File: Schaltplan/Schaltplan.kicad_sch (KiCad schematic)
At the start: 9 parts, among them J2 Buck Converter, M2 Stepper_Motor_bipolar, M3 Stepper_Motor_bipolar

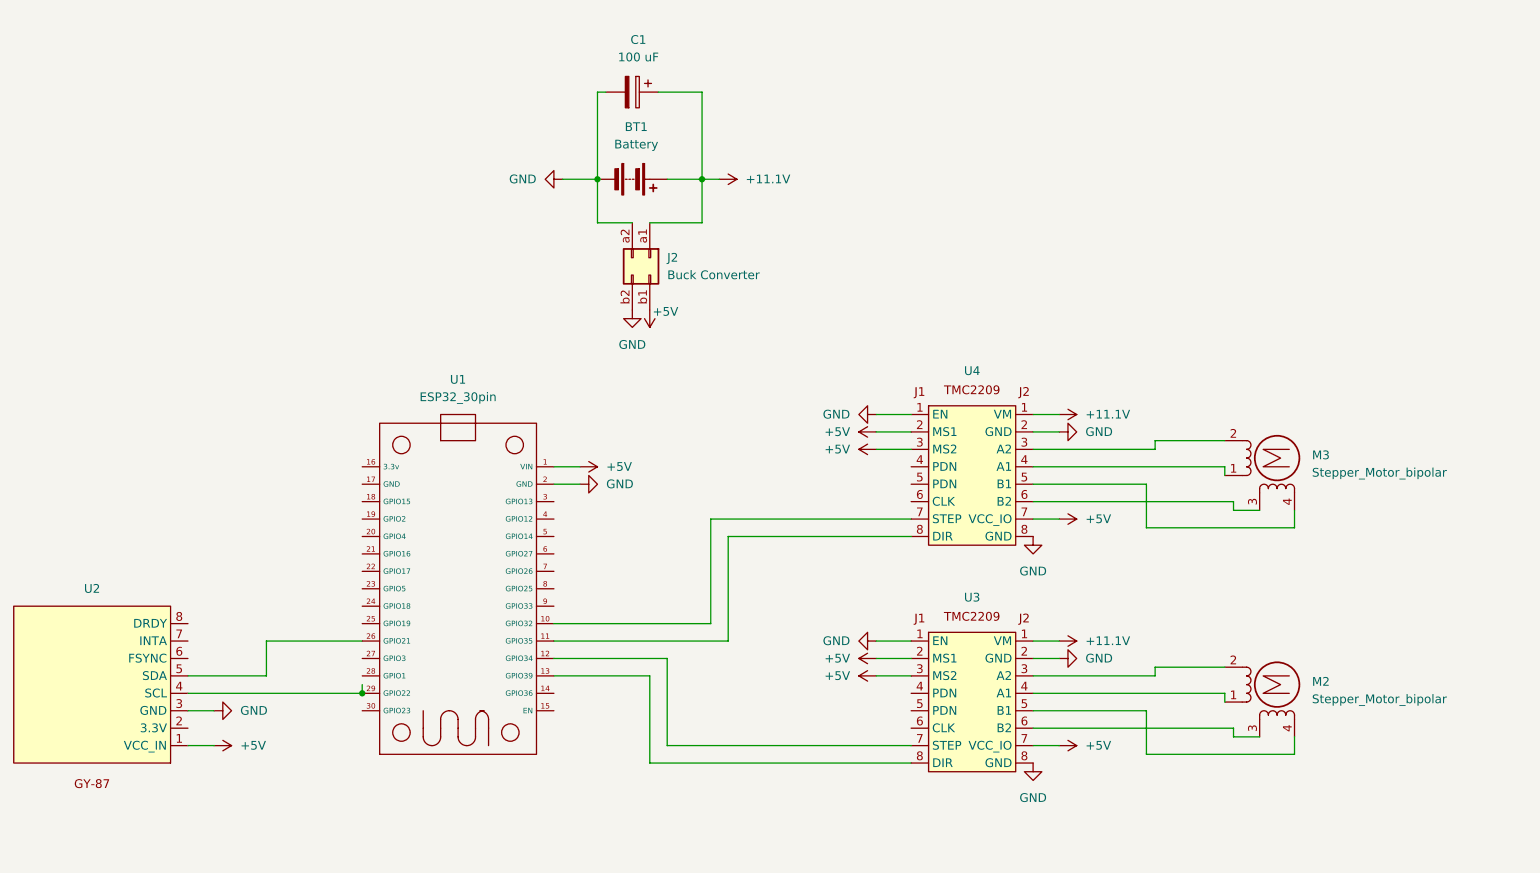
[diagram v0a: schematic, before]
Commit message: New file names
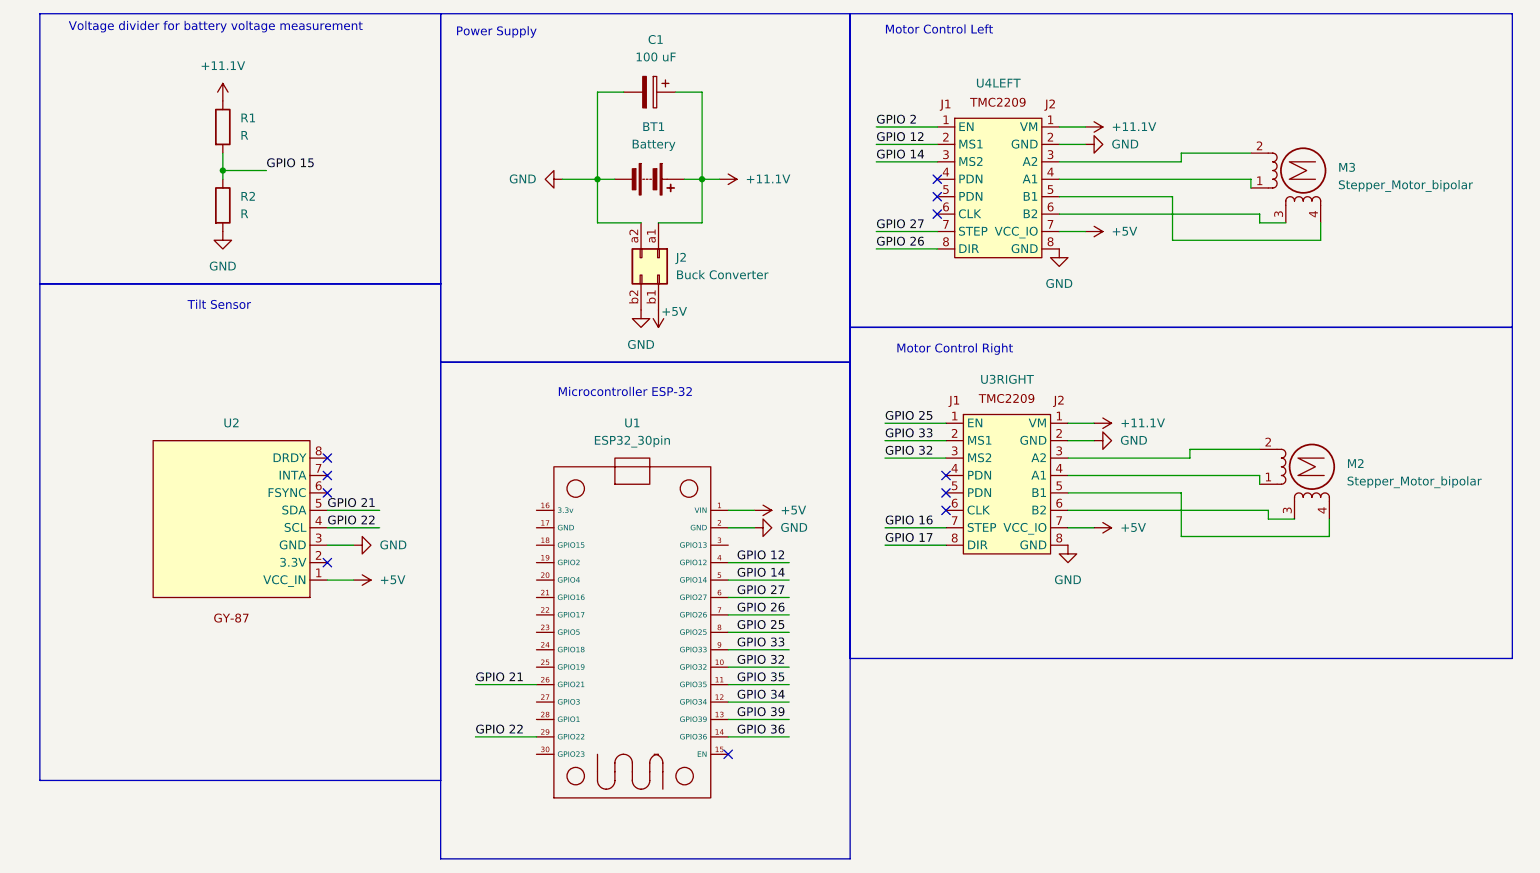
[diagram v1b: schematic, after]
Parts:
- added R1, R2: R, symbol Device:R
- renumbered U3 to U3RIGHT, U4 to U4LEFT
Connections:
- net +11.1V: now also R1.1
- net +5V: no longer U3RIGHT.2 (GND), U3RIGHT.3 (A2), U4LEFT.2 (GND), U4LEFT.3 (A2)
- net GND: now also R2.2; no longer U3RIGHT.1 (VM), U4LEFT.1 (VM)
- net at U3RIGHT.4 (A1): now also M2.1
- net at U3RIGHT.5 (B1): now also M2.4
- net at U3RIGHT.6 (B2): now also M2.3
- net GPIO 16: now reaches U3RIGHT.7 (VCC_IO)
- net GPIO 16: no longer U1.12 (GPIO34)
- net GPIO 17: now reaches U3RIGHT.8 (GND)
- net GPIO 17: no longer U1.13 (GPIO39)
- net at U4LEFT.4 (A1): now also M3.1
- net at U4LEFT.5 (B1): now also M3.4
- net at U4LEFT.6 (B2): now also M3.3
- net GPIO 27: now reaches U4LEFT.7 (VCC_IO)
- net GPIO 27: now also U1.6 (GPIO27); no longer U1.10 (GPIO32)
- net GPIO 26: now reaches U4LEFT.8 (GND)
- net GPIO 26: now also U1.7 (GPIO26); no longer U1.11 (GPIO35)
- net GPIO 36: now reaches U1.14 (GPIO36)
- net GPIO 21: now reaches U1.26 (GPIO21), U2.5 (SDA)
- net GPIO 22: now reaches U1.29 (GPIO22), U2.4 (SCL)
- net GPIO 12: now reaches U1.4 (GPIO12)
- net GPIO 12: now also U4LEFT.2 (GND)
- net GPIO 14: now reaches U1.5 (GPIO14)
- net GPIO 14: now also U4LEFT.3 (A2)
- net GPIO 25: now reaches U1.8 (GPIO25)
- net GPIO 25: now also U3RIGHT.1 (VM)
- net GPIO 33: now reaches U1.9 (GPIO33)
- net GPIO 33: now also U3RIGHT.2 (GND)
- new net GPIO 15: R1.2, R2.1
- new net GPIO 2: U4LEFT.1 (VM)
- new net GPIO 32: U1.10 (GPIO32), U3RIGHT.3 (A2)
- new net GPIO 34: U1.12 (GPIO34)
- new net GPIO 35: U1.11 (GPIO35)
- new net GPIO 39: U1.13 (GPIO39)
- no-connect marks 0 -> 11
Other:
- note added: "Microcontroller ESP-32"
- note added: "Motor Control Left"
- note added: "Motor Control Right"
- note added: "Power Supply"
- note added: "Tilt Sensor"
- note added: "Voltage divider for battery voltage measurement"
- moved on the sheet: BT1, C1, J2, M2, M3, U1, U2, U3RIGHT, U4LEFT
